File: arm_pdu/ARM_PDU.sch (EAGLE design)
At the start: 22 parts

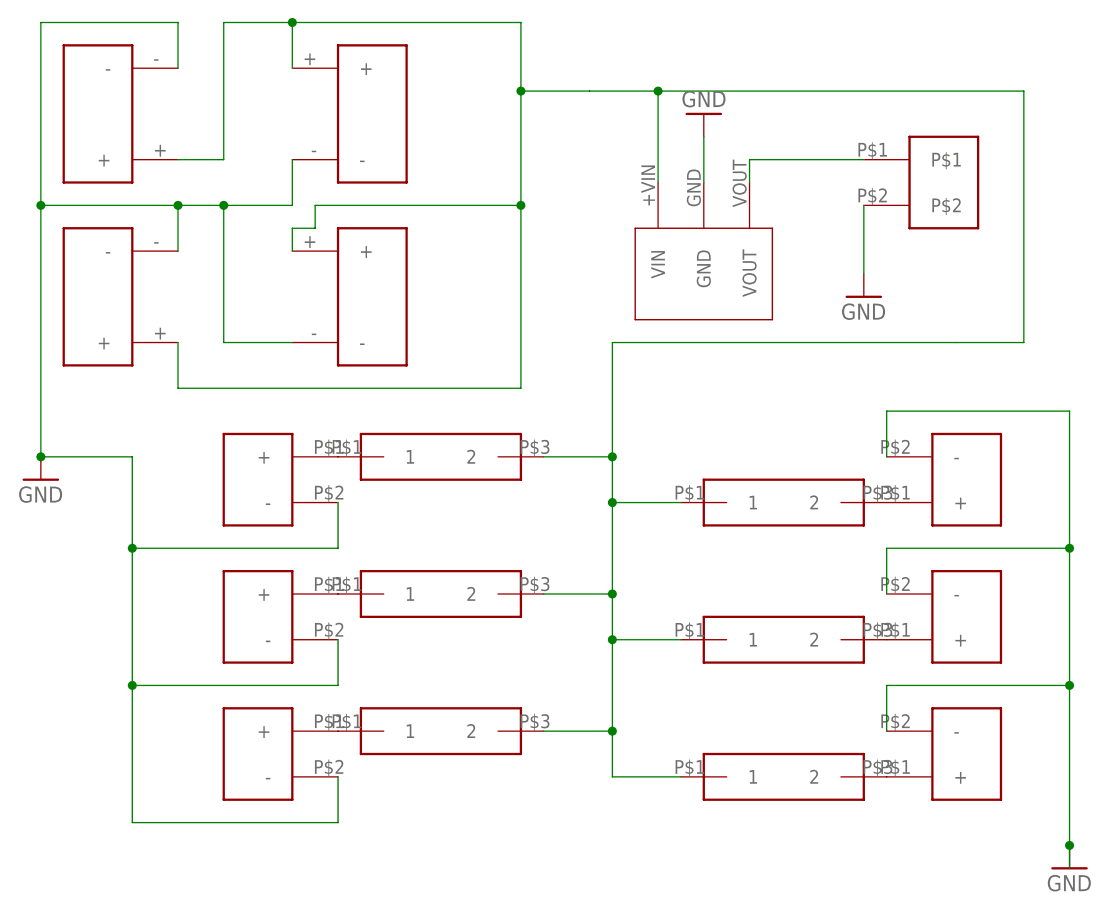
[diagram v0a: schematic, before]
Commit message: fixed issues with board not being in sync with schematic
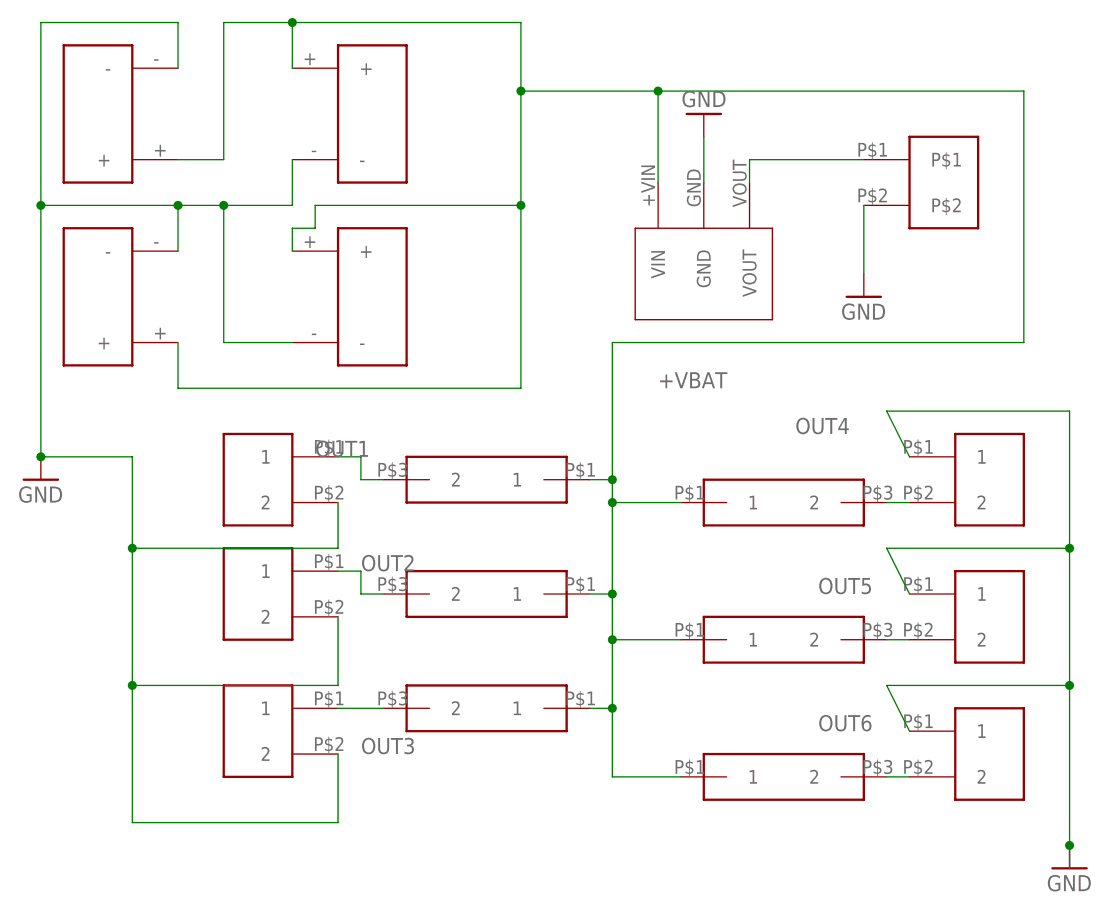
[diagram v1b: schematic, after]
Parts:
- removed 2PIN_CONNECTOR1, 2PIN_CONNECTOR2, 2PIN_CONNECTOR3, 2PIN_CONNECTOR4, 2PIN_CONNECTOR5, 2PIN_CONNECTOR6: 2PIN_CONNECTOR, 2PIN_CONNECTOR:2PIN_CONNECTOR
- added U$17, U$18: 2PIN_5MM, SPEAR-arm-pdu:2PIN_5MM
- U$10, U$11, U$12, U$13: value 20A_FUSE_HOLDER -> 2PIN_5MM; device 20A_FUSE_HOLDER:20A_FUSE_HOLDER -> SPEAR-arm-pdu:2PIN_5MM
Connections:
- removed net +VFUSED: U$1.2, U$14.1, U$15.1, U$16.1, U$2.2, U$3.2, U$4.+, U$5.+, U$6.+, U$7.+, U$9.VIN
- removed net N$1: 2PIN_CONNECTOR5.+, U$1.1
- removed net N$10: 2PIN_CONNECTOR3.+, U$15.2
- removed net N$11: 2PIN_CONNECTOR1.+, U$16.2
- removed net N$7: 2PIN_CONNECTOR4.+, U$2.1
- removed net N$8: 2PIN_CONNECTOR6.+, U$3.1
- removed net N$9: 2PIN_CONNECTOR2.+, U$14.2
- new net +VBAT: U$1.1, U$14.1, U$15.1, U$16.1, U$2.1, U$3.1, U$4.+, U$5.+, U$6.+, U$7.+, U$9.VIN
- new net OUT1: U$1.2, U$13.1
- new net OUT2: U$17.1, U$2.2
- new net OUT3: U$18.1, U$3.2
- new net OUT4: U$10.2, U$16.2
- new net OUT5: U$11.2, U$15.2
- new net OUT6: U$12.2, U$14.2
- net GND: now also U$10.1, U$11.1, U$12.1, U$13.2, U$17.2, U$18.2; no longer 2PIN_CONNECTOR1.-, 2PIN_CONNECTOR2.-, 2PIN_CONNECTOR3.-, 2PIN_CONNECTOR4.-, 2PIN_CONNECTOR5.-, 2PIN_CONNECTOR6.-
